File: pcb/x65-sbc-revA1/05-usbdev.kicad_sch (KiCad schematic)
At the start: 23 parts, among them J501 USB4085-GF-A, U503 74CBTLV3126PW,118, U504 FT2232HL, U601 SN74LVC1G08DBVR

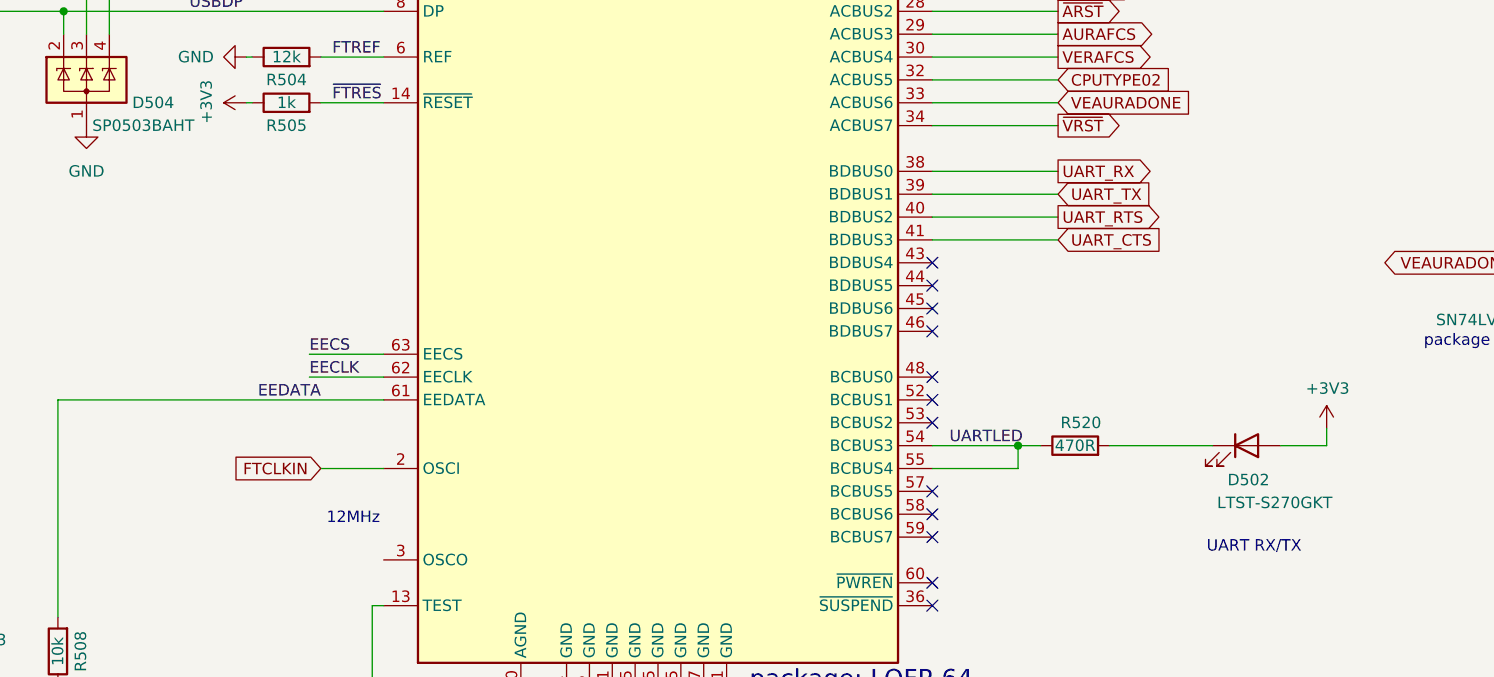
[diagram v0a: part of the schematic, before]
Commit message: pcb sbc: more pcb work
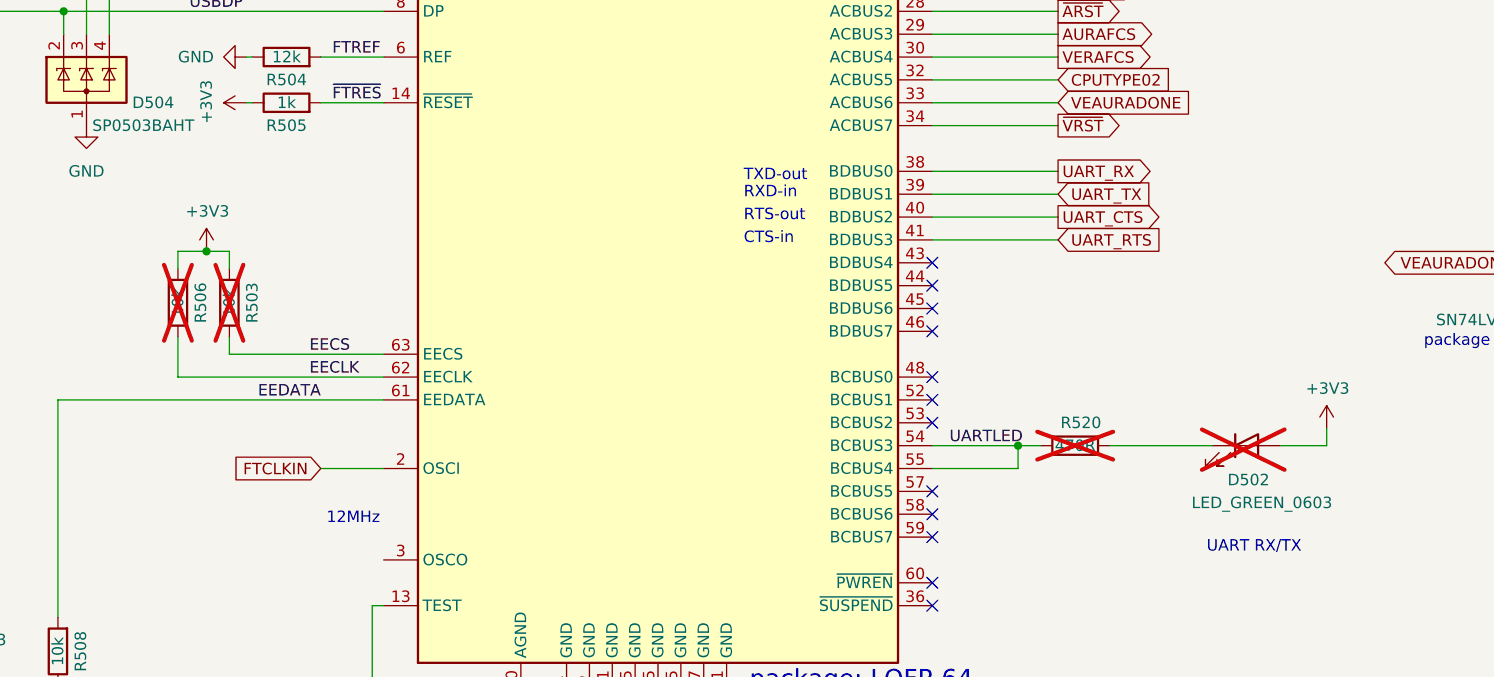
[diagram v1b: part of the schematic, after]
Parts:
- added R503, R506: 10k, Resistor_SMD:R_0603_1608Metric_Pad0.98x0.95mm_HandSolder, symbol Device:R
- D502: value LTST-S270GKT -> LED_GREEN_0603; now not fitted; now left out of the parts list
- R520: now not fitted; now left out of the parts list
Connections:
- net +3V3: now also R503.2, R506.2
- net EECLK: now also R506.1
- net EECS: now also R503.1
- net UART_CTS: now also U504.40 (BDBUS2); no longer U504.41 (BDBUS3)
- net UART_RTS: now also U504.41 (BDBUS3); no longer U504.40 (BDBUS2)
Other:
- note added: "CTS-in"
- note added: "RTS-out"
- note added: "RXD-in"
- note added: "TXD-out"
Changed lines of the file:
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@@
   (junction (at 59.69 90.805) (diameter 0) (color 0 0 0 0)
+  )
+  (junction (at 85.725 120.015) (diameter 0) (color 0 0 0 0)
   )
   (junction (at 130.81 172.085) (diameter 0) (color 0 0 0 0)
@@
     (stroke (width 0) (type default))
   )
-  (wire (pts (xy 97.155 133.985) (xy 105.41 133.985))
-    (stroke (width 0) (type default))
-  )
   (wire (pts (xy 138.43 172.085) (xy 140.97 172.085))
     (stroke (width 0) (type default))
@@
     (stroke (width 0) (type default))
   )
+  (wire (pts (xy 82.55 120.015) (xy 82.55 121.92))
+    (stroke (width 0) (type default))
+  )
+  (wire (pts (xy 88.265 131.445) (xy 105.41 131.445))
+    (stroke (width 0) (type default))
+  )
   (wire (pts (xy 133.35 169.545) (xy 133.35 172.085))
     (stroke (width 0) (type default))
@@
     (stroke (width 0) (type default))
   )
+  (wire (pts (xy 82.55 133.985) (xy 82.55 129.54))
+    (stroke (width 0) (type default))
+  )
   (wire (pts (xy 212.725 88.265) (xy 215.265 88.265))
     (stroke (width 0) (type default))
@@
     (stroke (width 0) (type default))
   )
+  (wire (pts (xy 88.265 131.445) (xy 88.265 129.54))
+    (stroke (width 0) (type default))
+  )
   (wire (pts (xy 200.66 70.485) (xy 240.665 70.485))
     (stroke (width 0) (type default))
@@
     (stroke (width 0) (type default))
   )
+  (wire (pts (xy 85.725 120.015) (xy 82.55 120.015))
+    (stroke (width 0) (type default))
+  )
+  (wire (pts (xy 82.55 133.985) (xy 105.41 133.985))
+    (stroke (width 0) (type default))
+  )
   (wire (pts (xy 130.81 55.245) (xy 130.81 57.785))
     (stroke (width 0) (type default))
@@
     (stroke (width 0) (type default))
   )
-  (wire (pts (xy 97.155 131.445) (xy 105.41 131.445))
-    (stroke (width 0) (type default))
-  )
   (wire (pts (xy 105.41 70.485) (xy 96.52 70.485))
     (stroke (width 0) (type default))
@@
     (stroke (width 0) (type default))
   )
+  (wire (pts (xy 85.725 120.015) (xy 88.265 120.015))
+    (stroke (width 0) (type default))
+  )
   (wire (pts (xy 130.81 169.545) (xy 130.81 172.085))
     (stroke (width 0) (type default))
@@
   )
   (wire (pts (xy 45.72 169.545) (xy 60.96 169.545))
+    (stroke (width 0) (type default))
+  )
+  (wire (pts (xy 88.265 120.015) (xy 88.265 121.92))
     (stroke (width 0) (type default))
   )
@@
     (effects (font (size 1.27 1.27)) (justify right bottom))
   )
+  (text "RTS-out" (at 145.415 116.84 0)
+    (effects (font (size 1.27 1.27)) (justify left bottom))
+  )
   (text "package: LQFP-64" (at 146.05 168.91 0)
     (effects (font (size 2 2)) (justify left bottom))
@@
     (effects (font (size 1.27 1.27)) (justify left bottom))
   )
+  (text "CTS-in" (at 145.415 119.38 0)
+    (effects (font (size 1.27 1.27)) (justify left bottom))
+  )
   (text "package: TSSOP-14" (at 216.535 59.69 0)
     (effects (font (size 1.27 1.27)) (justify left bottom))
   )
   (text "UART RX/TX" (at 196.85 153.67 0)
+    (effects (font (size 1.27 1.27)) (justify left bottom))
+  )
+  (text "RXD-in" (at 145.415 114.3 0)
+    (effects (font (size 1.27 1.27)) (justify left bottom))
+  )
+  (text "TXD-out" (at 145.415 112.395 0)
     (effects (font (size 1.27 1.27)) (justify left bottom))
   )
@@
     )
   )
-  (global_label "UART_RTS" (shape output) (at 180.34 116.205 0) (fields_autoplaced)
+  (global_label "UART_CTS" (shape output) (at 180.34 116.205 0) (fields_autoplaced)
     (effects (font (size 1.27 1.27)) (justify left))
-    (property "Intersheetrefs" "${INTERSHEET_REFS}" (at 191.8245 116.1256 0)
+    (property "Intersheetrefs" "${INTERSHEET_REFS}" (at 192.3966 116.205 0)
       (effects (font (size 1.27 1.27)) (justify left) hide)
     )
@@
     )
   )
-  (global_label "UART_CTS" (shape input) (at 180.34 118.745 0) (fields_autoplaced)
+  (global_label "UART_RTS" (shape input) (at 180.34 118.745 0) (fields_autoplaced)
     (effects (font (size 1.27 1.27)) (justify left))
-    (property "Intersheetrefs" "${INTERSHEET_REFS}" (at 191.8245 118.6656 0)
+    (property "Intersheetrefs" "${INTERSHEET_REFS}" (at 192.3966 118.745 0)
       (effects (font (size 1.27 1.27)) (justify left) hide)
     )
@@
         (path "/85750bea-43a1-4629-9575-611e72af7f9f/3a4f5a92-8b22-4d71-ac4e-37e2fe30ebbe"
           (reference "D501") (unit 1)
+        )
+      )
+    )
+  )
+  (symbol (lib_id "Device:R") (at 82.55 125.73 180) (unit 1)
+    (in_bom no) (on_board yes) (dnp yes)
+    (property "Reference" "R506" (at 85.09 125.73 90)
+      (effects (font (size 1.27 1.27)))
+    )
+    (property "Value" "10k" (at 82.55 125.73 90)
+      (effects (font (size 1.27 1.27)))
+    )
+    (property "Footprint" "Resistor_SMD:R_0603_1608Metric_Pad0.98x0.95mm_HandSolder" (at 84.328 125.73 90)
+      (effects (font (size 1.27 1.27)) hide)
+    )
+    (property "Datasheet" "~" (at 82.55 125.73 0)
+      (effects (font (size 1.27 1.27)) hide)
+    )
+    (pin "1")
+    (pin "2")
+    (instances
+      (project "x65-sbc-revA1"
+        (path "/85750bea-43a1-4629-9575-611e72af7f9f/3a4f5a92-8b22-4d71-ac4e-37e2fe30ebbe"
+          (reference "R506") (unit 1)
         )
       )
@@
   )
   (symbol (lib_id "Device:R") (at 182.245 141.605 90) (unit 1)
-    (in_bom yes) (on_board yes) (dnp no)
+    (in_bom no) (on_board yes) (dnp yes)
     (property "Reference" "R520" (at 182.88 139.065 90)
       (effects (font (size 1.27 1.27)))
@@
   )
   (symbol (lib_id "Device:LED") (at 201.295 141.605 0) (unit 1)
-    (in_bom yes) (on_board yes) (dnp no)
+    (in_bom no) (on_board yes) (dnp yes)
     (property "Reference" "D502" (at 203.835 145.415 0)
       (effects (font (size 1.27 1.27)) (justify right))
     )
-    (property "Value" "LTST-S270GKT" (at 210.82 147.955 0)
+    (property "Value" "LED_GREEN_0603" (at 210.82 147.955 0)
       (effects (font (size 1.27 1.27)) (justify right))
     )
@@
         (path "/85750bea-43a1-4629-9575-611e72af7f9f/3a4f5a92-8b22-4d71-ac4e-37e2fe30ebbe"
           (reference "#PWR0508") (unit 1)
+        )
+      )
+    )
+  )
+  (symbol (lib_id "power:+3V3") (at 85.725 120.015 0) (unit 1)
+    (in_bom yes) (on_board yes) (dnp no)
+    (property "Reference" "#PWR0510" (at 85.725 123.825 0)
+      (effects (font (size 1.27 1.27)) hide)
+    )
+    (property "Value" "+3V3" (at 88.265 115.57 0)
+      (effects (font (size 1.27 1.27)) (justify right))
+    )
+    (property "Footprint" "" (at 85.725 120.015 0)
+      (effects (font (size 1.27 1.27)) hide)
+    )
+    (property "Datasheet" "" (at 85.725 120.015 0)
+      (effects (font (size 1.27 1.27)) hide)
+    )
+    (pin "1")
+    (instances
+      (project "x65-sbc-revA1"
+        (path "/85750bea-43a1-4629-9575-611e72af7f9f/3a4f5a92-8b22-4d71-ac4e-37e2fe30ebbe"
+          (reference "#PWR0510") (unit 1)
         )
       )
@@
         )
       )
+    )
+  )
+  (symbol (lib_id "Device:R") (at 88.265 125.73 180) (unit 1)
+    (in_bom no) (on_board yes) (dnp yes)
+    (property "Reference" "R503" (at 90.805 125.73 90)
+      (effects (font (size 1.27 1.27)))
+    )
+    (property "Value" "10k" (at 88.265 125.73 90)
+      (effects (font (size 1.27 1.27)))
+    )
+    (property "Footprint" "Resistor_SMD:R_0603_1608Metric_Pad0.98x0.95mm_HandSolder" (at 90.043 125.73 90)
+      (effects (font (size 1.27 1.27)) hide)
+    )
+    (property "Datasheet" "~" (at 88.265 125.73 0)
+      (effects (font (size 1.27 1.27)) hide)
+    )
+    (pin "1")
+    (pin "2")
+    (instances
+      (project "x65-sbc-revA1"
+        (path "/85750bea-43a1-4629-9575-611e72af7f9f/3a4f5a92-8b22-4d71-ac4e-37e2fe30ebbe"
+          (reference "R503") (unit 1)
+        )
+      )
